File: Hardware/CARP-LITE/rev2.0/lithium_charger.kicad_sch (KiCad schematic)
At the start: 23 parts, among them U1 BQ25792

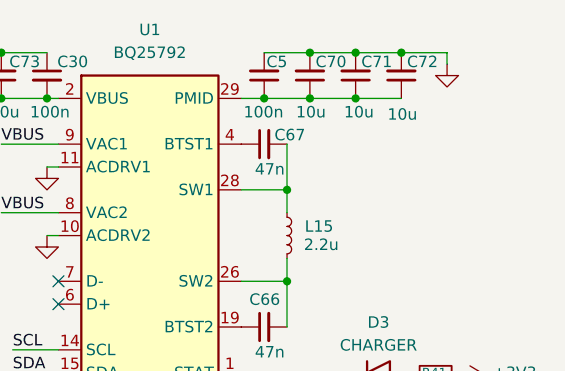
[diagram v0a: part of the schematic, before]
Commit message: powersection
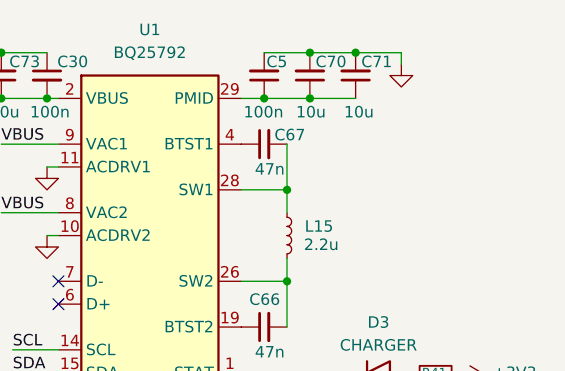
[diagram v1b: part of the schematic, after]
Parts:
- removed C72: 10u, Capacitor_SMD:C_0805_2012Metric, symbol Device:C_Small
- C69: footprint Capacitor_SMD:C_0603_1608Metric -> Capacitor_SMD:C_0402_1005Metric
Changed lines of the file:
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@@
-	)
-	(junction
-		(at 172.72 71.12)
-		(diameter 0)
-		(color 0 0 0 0)
 	)
 	(junction
@@
 		(color 0 0 0 0)
 	)
-	(junction
-		(at 177.8 66.04)
-		(diameter 0)
-		(color 0 0 0 0)
-	)
 	(no_connect
 		(at 139.7 91.44)
@@
 	(wire
 		(pts
-			(xy 177.8 66.04) (xy 172.72 66.04)
+			(xy 172.72 66.04) (xy 177.8 66.04)
 		)
 		(stroke
@@
 	(wire
 		(pts
-			(xy 172.72 71.12) (xy 177.8 71.12)
-		)
-		(stroke
-			(width 0)
-			(type default)
-		)
-	)
-	(wire
-		(pts
 			(xy 160.02 127) (xy 161.29 127)
 		)
@@
 	(wire
 		(pts
-			(xy 182.88 66.04) (xy 182.88 67.31)
+			(xy 177.8 66.04) (xy 177.8 67.31)
 		)
 		(stroke
@@
 		(pts
 			(xy 133.35 66.04) (xy 138.43 66.04)
-		)
-		(stroke
-			(width 0)
-			(type default)
-		)
-	)
-	(wire
-		(pts
-			(xy 177.8 66.04) (xy 182.88 66.04)
 		)
 		(stroke
@@
 			)
 		)
-		(property "Footprint" "Capacitor_SMD:C_0603_1608Metric"
+		(property "Footprint" "Capacitor_SMD:C_0402_1005Metric"
 			(at 162.56 121.92 0)
 			(hide yes)
@@
 	(symbol
 		(lib_id "power:GND")
-		(at 182.88 67.31 0)
+		(at 177.8 67.31 0)
 		(unit 1)
 		(body_style 1)
@@
 		(dnp no)
 		(property "Reference" "#PWR0118"
-			(at 182.88 73.66 0)
+			(at 177.8 73.66 0)
 			(hide yes)
 			(show_name no)
@@
 		)
 		(property "Value" "GND"
-			(at 183.007 71.7042 0)
+			(at 177.927 71.7042 0)
 			(hide yes)
 			(show_name no)
@@
 		)
 		(property "Footprint" ""
-			(at 182.88 67.31 0)
+			(at 177.8 67.31 0)
 			(hide yes)
 			(show_name no)
@@
 		)
 		(property "Datasheet" ""
-			(at 182.88 67.31 0)
+			(at 177.8 67.31 0)
 			(hide yes)
 			(show_name no)
@@
 		)
 		(property "Description" ""
-			(at 182.88 67.31 0)
+			(at 177.8 67.31 0)
 			(show_name no)
 			(do_not_autoplace no)
@@
 					(unit 1)
 				)
-			)
-		)
-	)
-	(symbol
-		(lib_id "Device:C_Small")
-		(at 177.8 68.58 180)
-		(unit 1)
-		(body_style 1)
-		(exclude_from_sim no)
-		(in_bom yes)
-		(on_board yes)
-		(in_pos_files yes)
-		(dnp no)
-		(property "Reference" "C72"
-			(at 181.864 67.056 0)
-			(show_name no)
-			(do_not_autoplace no)
-			(effects
-				(font
-					(size 1.27 1.27)
-				)
-				(justify left)
-			)
-		)
-		(property "Value" "10u"
-			(at 179.578 72.898 0)
-			(show_name no)
-			(do_not_autoplace no)
-			(effects
-				(font
-					(size 1.27 1.27)
-				)
-				(justify left)
-			)
-		)
-		(property "Footprint" "Capacitor_SMD:C_0805_2012Metric"
-			(at 177.8 68.58 0)
-			(hide yes)
-			(show_name no)
-			(do_not_autoplace no)
-			(effects
-				(font
-					(size 1.27 1.27)
-				)
-			)
-		)
-		(property "Datasheet" ""
-			(at 177.8 68.58 0)
-			(hide yes)
-			(show_name no)
-			(do_not_autoplace no)
-			(effects
-				(font
-					(size 1.27 1.27)
-				)
-			)
-		)
-		(property "Description" "Unpolarized capacitor, small symbol"
-			(at 177.8 68.58 0)
-			(hide yes)
-			(show_name no)
-			(do_not_autoplace no)
-			(effects
-				(font
-					(size 1.27 1.27)
-				)
-			)
-		)
-		(pin "2"
-		)
-		(pin "1"
-		)
-		(instances
-			(project "CARP"
-				(path "/94683f5c-9cd9-448e-be96-9792537b5cb8/4876be96-b063-438e-9f90-27783f3ee277"
-					(reference "C72")
-					(unit 1)
-				)
